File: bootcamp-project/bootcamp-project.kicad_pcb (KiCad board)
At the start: 2 copper layers, 26.8 x 33.5 mm, 18 parts, among them J3 FTDI, SW1 SW_Push, U1 ATmega328P-A, Y1 16MHz

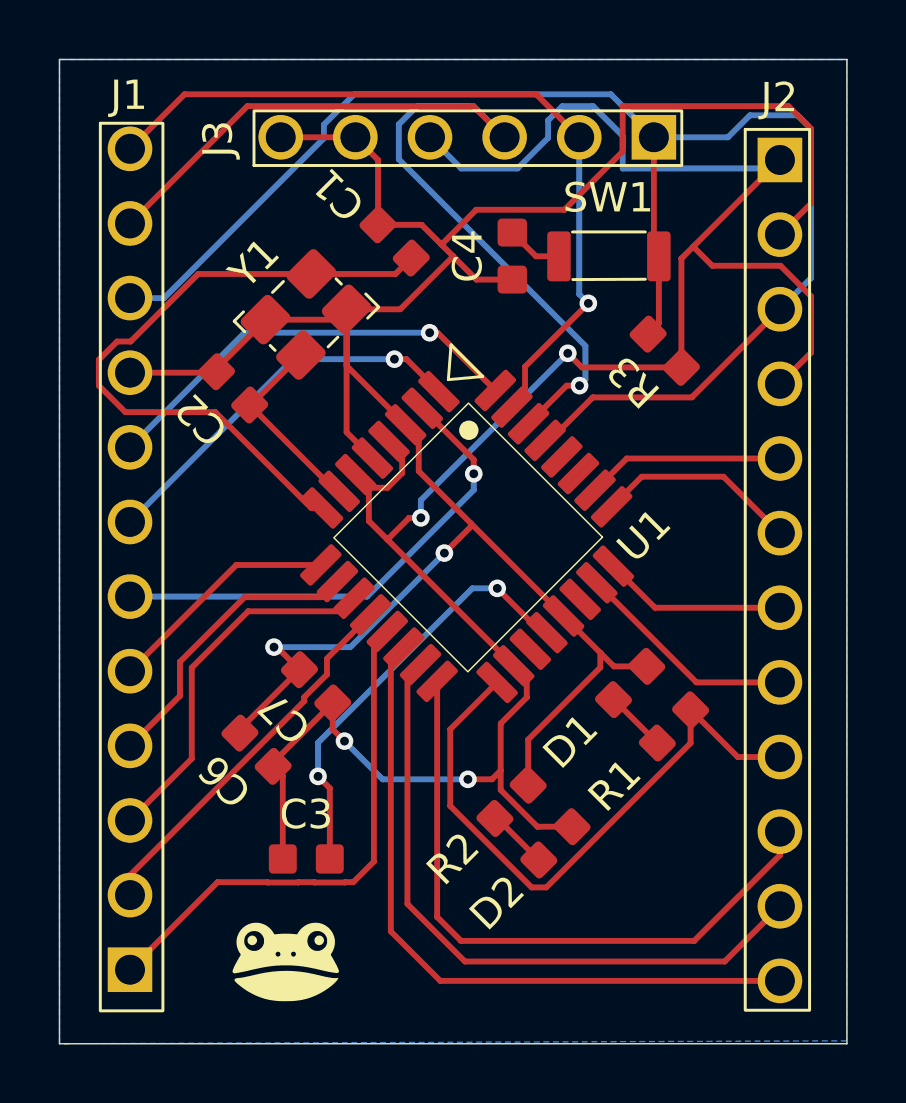
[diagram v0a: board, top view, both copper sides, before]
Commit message: add: bonuses
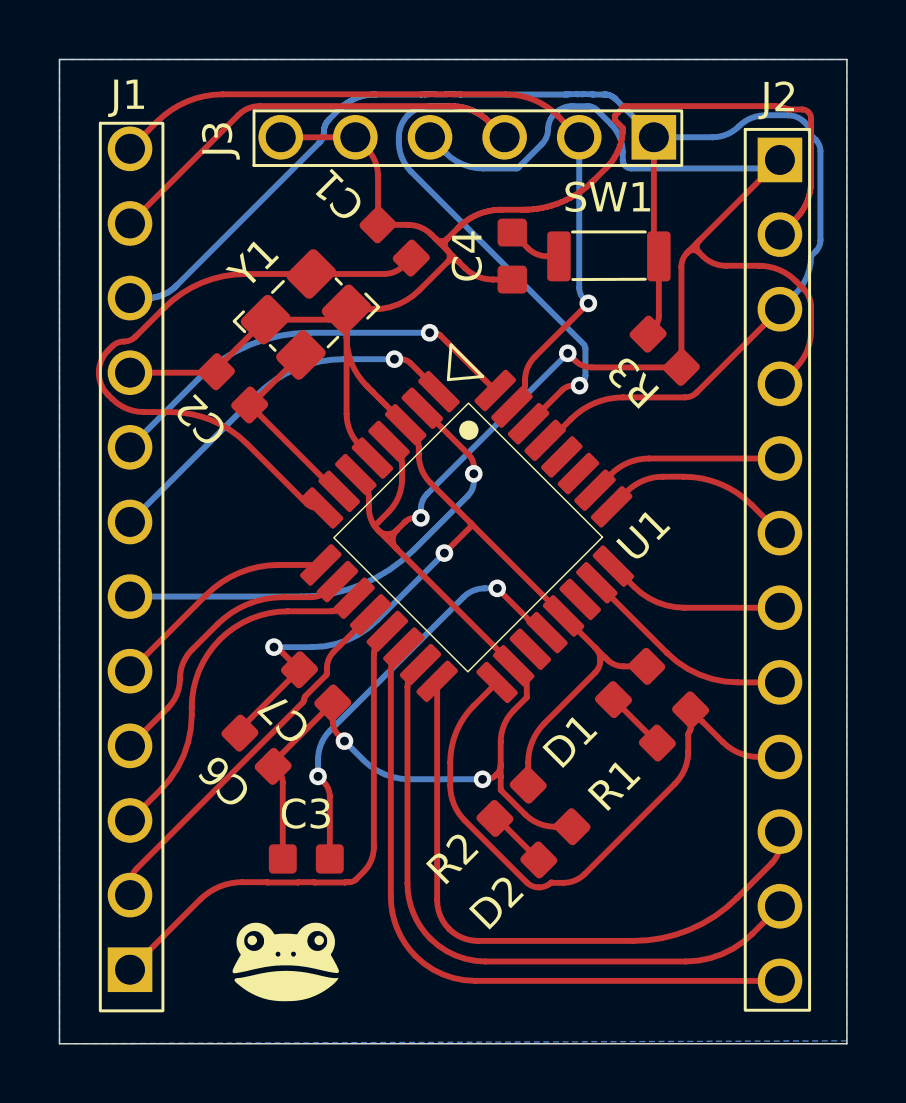
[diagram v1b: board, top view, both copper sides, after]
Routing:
- net RAW: track 77.8 -> 78.6 mm
- net GND: track 84.4 -> 85.2 mm
- net Net-(U1-XTAL2/PB7): track 22.3 -> 21.6 mm
- net SCK: track 21.1 -> 20.5 mm
- net D7: track 12.6 -> 12.0 mm
